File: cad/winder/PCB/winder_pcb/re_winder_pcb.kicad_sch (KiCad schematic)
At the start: 33 parts, among them J1 12V_IN, M1 Motor_DC

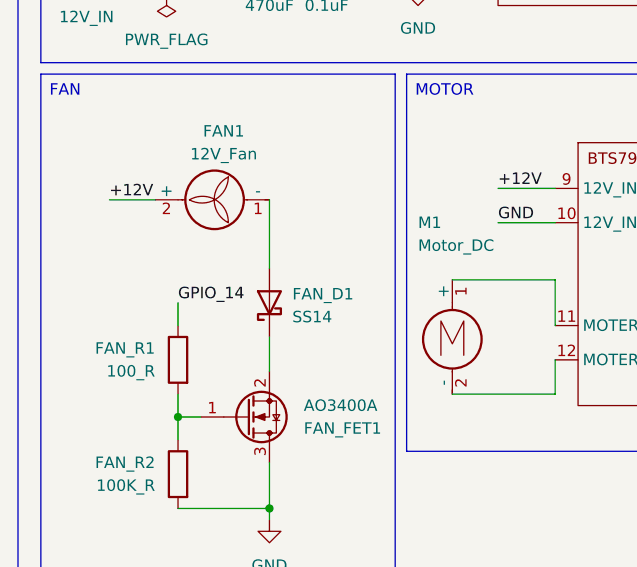
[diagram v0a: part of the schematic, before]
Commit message: パワー基盤の作成完了
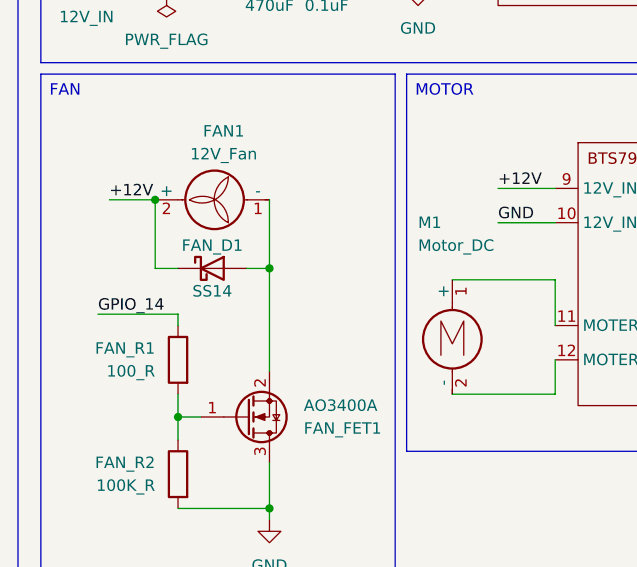
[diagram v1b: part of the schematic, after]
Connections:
- net +12V: now also FAN_D1.1 (K)
- net at FAN_FET1.2 (S): now also FAN1.1 (-), FAN_D1.2 (A); no longer FAN_D1.1 (K)
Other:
- moved on the sheet: FAN_D1
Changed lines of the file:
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@@
 	)
 	(junction
+		(at 55.88 69.85)
+		(diameter 0)
+		(color 0 0 0 0)
+	)
+	(junction
 		(at 195.58 157.48)
 		(diameter 0)
@@
 		(color 0 0 0 0)
 	)
+	(junction
+		(at 43.18 62.23)
+		(diameter 0)
+		(color 0 0 0 0)
+	)
 	(no_connect
 		(at 175.26 72.39)
@@
 	(wire
 		(pts
-			(xy 55.88 77.47) (xy 55.88 81.28)
-		)
-		(stroke
-			(width 0)
-			(type default)
-		)
-	)
-	(wire
-		(pts
 			(xy 55.88 91.44) (xy 55.88 96.52)
 		)
@@
 	(wire
 		(pts
+			(xy 45.72 74.93) (xy 45.72 76.2)
+		)
+		(stroke
+			(width 0)
+			(type default)
+		)
+	)
+	(wire
+		(pts
 			(xy 166.37 123.19) (xy 176.53 123.19)
 		)
@@
 	(wire
 		(pts
+			(xy 45.72 69.85) (xy 43.18 69.85)
+		)
+		(stroke
+			(width 0)
+			(type default)
+		)
+	)
+	(wire
+		(pts
+			(xy 55.88 69.85) (xy 55.88 81.28)
+		)
+		(stroke
+			(width 0)
+			(type default)
+		)
+	)
+	(wire
+		(pts
 			(xy 44.45 35.56) (xy 52.07 35.56)
 		)
@@
 	(wire
 		(pts
-			(xy 245.11 113.03) (xy 248.92 113.03)
+			(xy 43.18 69.85) (xy 43.18 62.23)
 		)
 		(stroke
@@
 	(wire
 		(pts
-			(xy 240.03 147.32) (xy 240.03 152.4)
+			(xy 245.11 113.03) (xy 248.92 113.03)
 		)
 		(stroke
@@
 	(wire
 		(pts
-			(xy 168.91 146.05) (xy 176.53 146.05)
+			(xy 240.03 147.32) (xy 240.03 152.4)
 		)
 		(stroke
@@
 	(wire
 		(pts
-			(xy 45.72 96.52) (xy 55.88 96.52)
+			(xy 168.91 146.05) (xy 176.53 146.05)
 		)
 		(stroke
@@
 	(wire
 		(pts
-			(xy 116.84 30.48) (xy 116.84 35.56)
+			(xy 45.72 96.52) (xy 55.88 96.52)
 		)
 		(stroke
@@
 	(wire
 		(pts
-			(xy 55.88 62.23) (xy 55.88 69.85)
+			(xy 116.84 30.48) (xy 116.84 35.56)
 		)
 		(stroke
@@
 	(wire
 		(pts
-			(xy 45.72 73.66) (xy 45.72 76.2)
+			(xy 55.88 62.23) (xy 55.88 69.85)
 		)
 		(stroke
@@
 	(wire
 		(pts
+			(xy 53.34 69.85) (xy 55.88 69.85)
+		)
+		(stroke
+			(width 0)
+			(type default)
+		)
+	)
+	(wire
+		(pts
 			(xy 204.47 73.66) (xy 207.01 73.66)
 		)
@@
 	(wire
 		(pts
+			(xy 36.83 74.93) (xy 45.72 74.93)
+		)
+		(stroke
+			(width 0)
+			(type default)
+		)
+	)
+	(wire
+		(pts
 			(xy 193.04 154.94) (xy 194.31 154.94)
 		)
@@
 	)
 	(label "GPIO_14"
-		(at 45.72 73.66 0)
+		(at 36.83 74.93 0)
 		(effects
 			(font
@@
 	(symbol
 		(lib_id "Diode:SS14")
-		(at 55.88 73.66 90)
+		(at 49.53 69.85 0)
 		(unit 1)
 		(exclude_from_sim no)
@@
 		(on_board yes)
 		(dnp no)
-		(fields_autoplaced yes)
 		(property "Reference" "FAN_D1"
-			(at 58.42 72.7074 90)
+			(at 49.53 67.31 0)
 			(effects
 				(font
 					(size 1.27 1.27)
 				)
-				(justify right)
 			)
 		)
 		(property "Value" "SS14"
-			(at 58.42 75.2474 90)
+			(at 49.53 72.39 0)
 			(effects
 				(font
 					(size 1.27 1.27)
 				)
-				(justify right)
 			)
 		)
 		(property "Footprint" "Diode_SMD:D_SMA"
-			(at 60.325 73.66 0)
+			(at 49.53 74.295 0)
 			(effects
 				(font
@@
 		)
 		(property "Datasheet" "https://www.vishay.com/docs/88746/ss12.pdf"
-			(at 55.88 73.66 0)
+			(at 49.53 69.85 0)
 			(effects
 				(font
@@
 		)
 		(property "Description" "40V 1A Schottky Diode, SMA"
-			(at 55.88 73.66 0)
+			(at 49.53 69.85 0)
 			(effects
 				(font
